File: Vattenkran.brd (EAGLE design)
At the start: 100 x 80 mm, 28 parts, among them J1 Battery, J2 Solar, J3 Valve, J4 Wakeup Button, Q2 32KHz

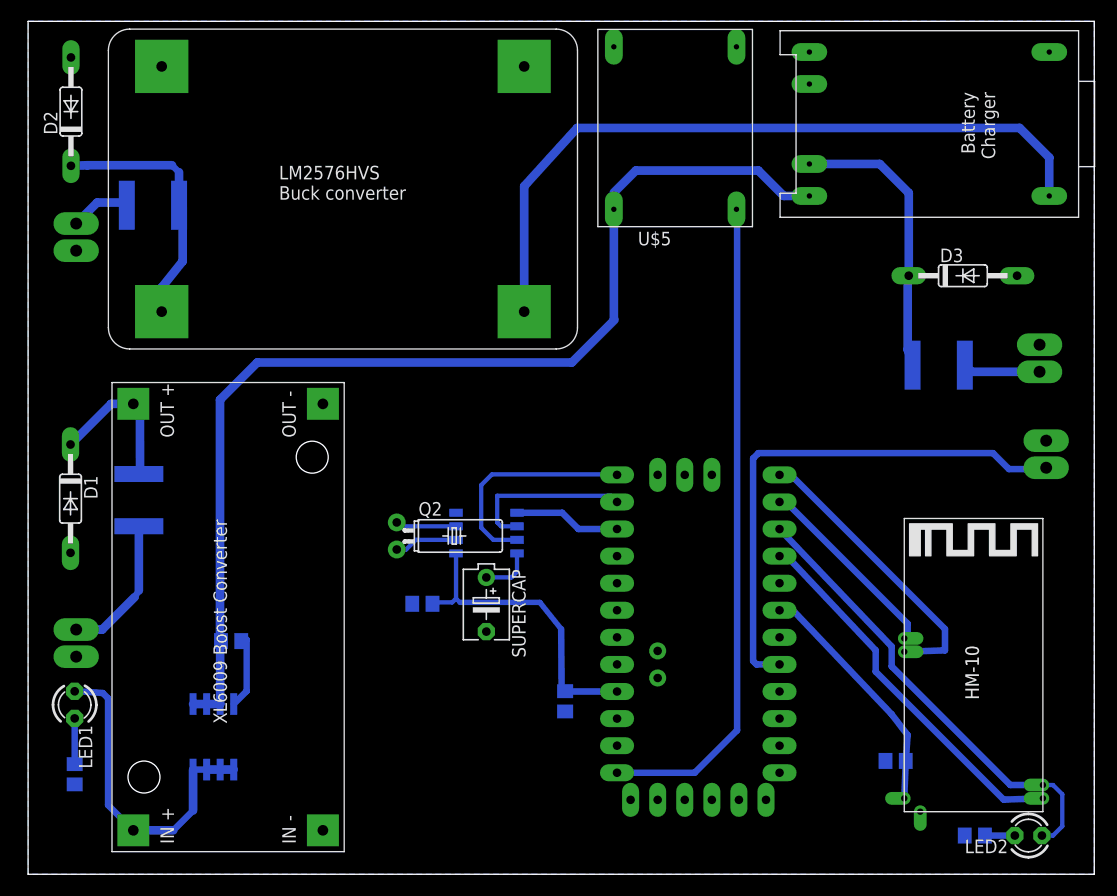
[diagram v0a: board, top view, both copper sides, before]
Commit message: Layout
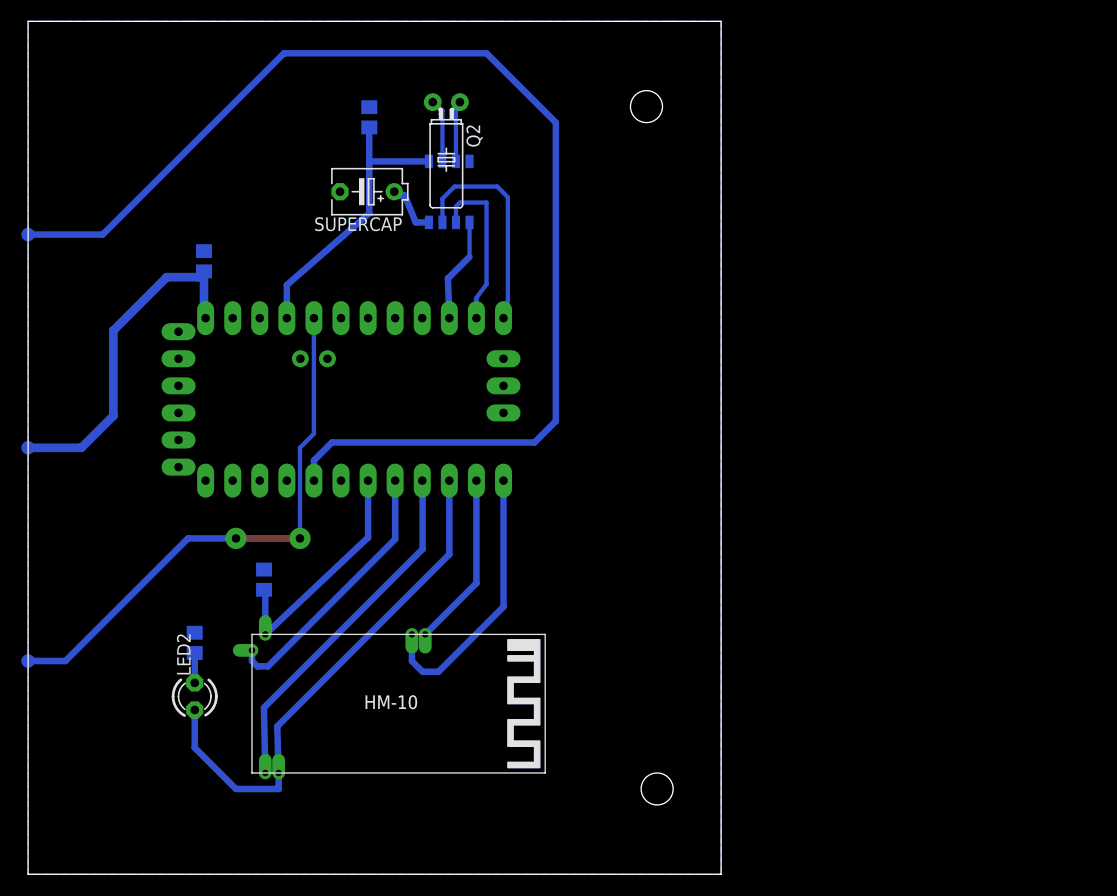
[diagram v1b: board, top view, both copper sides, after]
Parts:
- removed D1, D2, D3: BAT19, diode:DO35-10
- removed J1: Battery, SparkFun-Connectors:1X02_LONGPADS
- removed J2: Solar, SparkFun-Connectors:1X02_LONGPADS
- removed J3: Valve, SparkFun-Connectors:1X02_LONGPADS
- removed J4: Wakeup Button, SparkFun-Connectors:1X02_LONGPADS
- removed LED1: GREEN, led:LED3MM
- removed R1: 1M, resistor:R0805
- removed R3: 3K3, resistor:R0805
- removed U$10: 500mA, fuse:MF-SMDF050
- removed U$11, U$3: MF-SMDF150, fuse:MF-SMDF050
- removed U$2: BATTERY_CHARGER, breakout-modules:BATTERY_CHARGER
- removed U$5: QSKJ_BOOST_MODULE, breakout-modules:QSKJ_BOOST_MODULE
- removed U$6: XL6009_BOOST_MODULE, breakout-modules:XL6009_BOOST_MODULE
- removed U$8: LM2576HVS_BUCK_MODULE, breakout-modules:LM2576HVS_BUCK_MODULE
- removed U$9: FDS6675, Semiconductors:SO08
- added TP1, TP2, TP3: TPB1,27, testpad:B1,27
- moved LED2 79.3 mm to (15.6, 16.7), turned to 90 degrees
- moved R2 75.4 mm to (15.6, 21.7), turned to 90 degrees
- moved U$4 68.4 mm to (21.0, 16.0), turned to 270 degrees
- moved C2 61.6 mm to (22.1, 27.6), turned to 90 degrees
- moved C3 53.4 mm to (16.5, 57.5), turned to 90 degrees
- moved U$7 49.8 mm to (23.0, 42.0), turned to 90 degrees
- moved C1 45.9 mm to (32.0, 71.0), turned to 90 degrees
- moved Q2 41.0 mm to (39.2, 72.4), turned to 180 degrees
- moved SUPERCAP 40.3 mm to (31.8, 64.0), turned to 180 degrees
- moved U$1 32.2 mm to (39.5, 64.0), turned to 180 degrees
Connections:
- removed net BT_POWER_ENABLE: R1.2, U$9.4
- removed net N$1: D2.C, U$10.2, U$8.IN
- removed net N$2: U$2.V_IN, U$8.OUT
- removed net N$36: D3.C, U$11.2, U$2.V_BATT+
- removed net N$6: D1.C, U$3.1, U$6.V_OUT
- removed net N$9: LED1.K, R3.1
- removed net SOLAR: J2.2, U$10.1
- removed net VALVE: J3.2, U$3.2
- removed net V_BATT+: J1.2, U$11.1
- removed net V_UNREG: R1.1, U$2.V_OUT, U$5.V_IN, U$9.1, U$9.2, U$9.3
- removed net V_VALVE_UNREG: LED1.A, U$6.V_IN, U$9.5, U$9.6, U$9.7, U$9.8
- new net VALVE_ENABLE: TP2.TP, U$7.A0
- net BUTTON_WAKEUP_INT: now also TP3.TP; no longer J4.2
- net GND: no longer D1.A, D2.A, D3.A, J1.1, J2.1, J3.1, J4.1, R3.2, U$2.GND@1, U$2.GND@2, U$2.V_BATT-, U$5.GND@1, U$5.GND@2, U$6.V_IN_GND, U$6.V_OUT_GND, U$8.GND@1, U$8.GND@2
- net VCC33: no longer C3.1
- net VCC5: now also C3.1, TP1.TP; no longer U$5.V_OUT
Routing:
- net V_UNREG: track 103.4 -> 0.00 mm
- net N$2: track 68.6 -> 0.00 mm
- net BUTTON_WAKEUP_INT: track 50.7 -> 113.3 mm
- net VALVE_ENABLE: track 0.00 -> 52.3 mm, vias 0 -> 2
- net V_VALVE_UNREG: track 30.7 -> 0.00 mm
- net VCC5: track 61.8 -> 32.5 mm
- net N$36: track 26.7 -> 0.00 mm
- net BT_GND: track 0.00 -> 25.1 mm
- net N$1: track 24.4 -> 0.00 mm
- net N$6: track 14.3 -> 0.00 mm
- net VALVE: track 13.5 -> 0.00 mm
- net V_BATT+: track 7.27 -> 0.00 mm
- net BT_POWER_ENABLE: track 7.10 -> 0.00 mm
- net SOLAR: track 5.61 -> 0.00 mm
- net BT_STATE: track 43.3 -> 48.6 mm
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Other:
- board size 100 x 80 mm -> 65 x 80 mm
